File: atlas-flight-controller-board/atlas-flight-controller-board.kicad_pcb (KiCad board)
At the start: 4 copper layers, 55.6 x 67.6 mm, 36 parts, among them IC1 LSM6DSV80XTR, IC2 LPS22HHTR, J1 LED Indicator Header, J4 5V Input Power, U1 LIS2MDL, U2 DEV-16771, U3 746

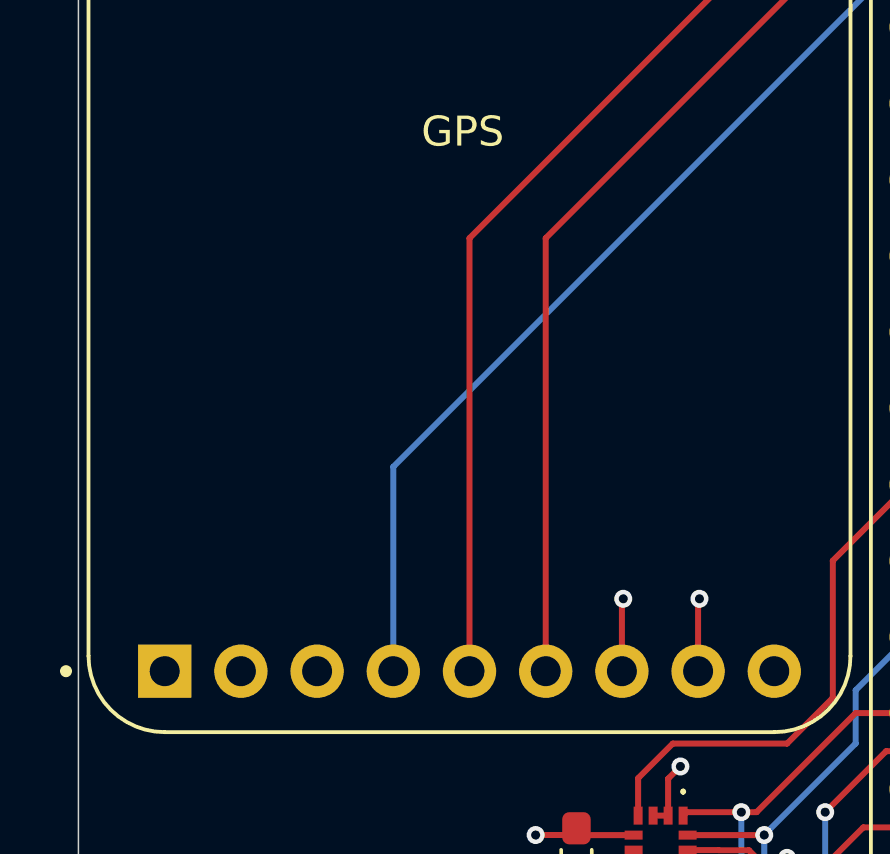
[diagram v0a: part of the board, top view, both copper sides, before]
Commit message: Test
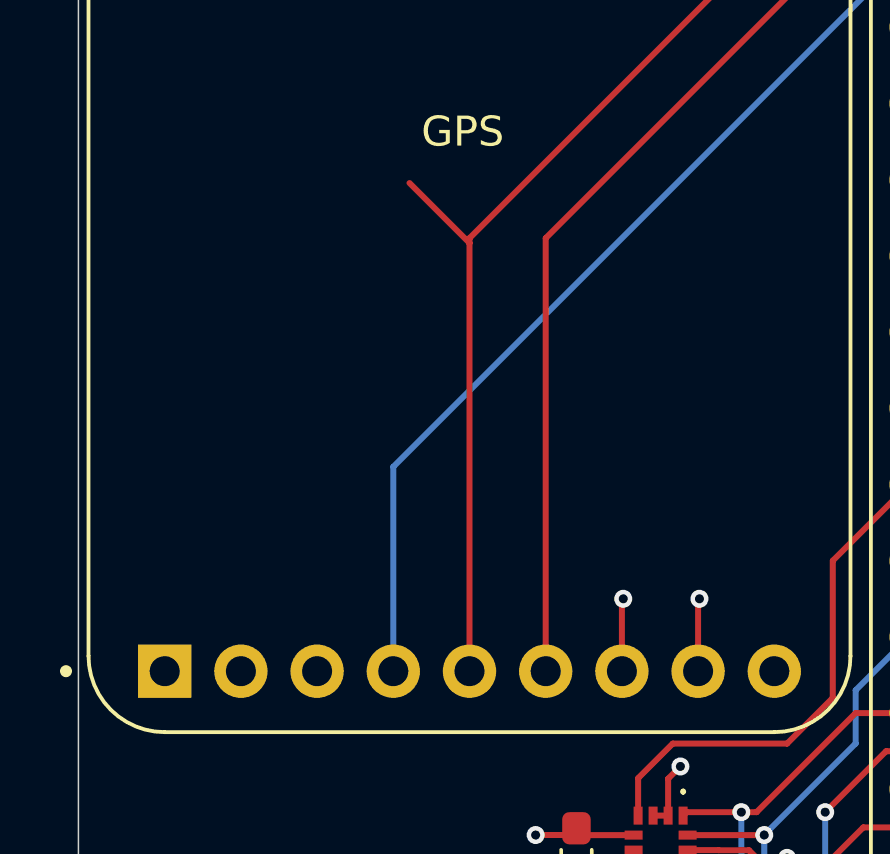
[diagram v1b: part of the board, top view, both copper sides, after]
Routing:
- net UART_GPS_TX_MCU_RX: track 35.2 -> 38.0 mm
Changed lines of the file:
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@@
 	)
 	(segment
-		(start 106 88.773)
+		(start 106 74.5)
 		(end 106 74.34)
+		(width 0.2)
+		(layer "F.Cu")
+		(net 9)
+	)
+	(segment
+		(start 106 74.5)
+		(end 104 72.5)
 		(width 0.2)
 		(layer "F.Cu")
@@
 		(width 0.2)
 		(layer "F.Cu")
+		(net 9)
+	)
+	(segment
+		(start 106 88.773)
+		(end 106 74.5)
+		(width 0.2)
+		(layer "F.Cu")

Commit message: testing commit on new branch made by kicad. branch name: version2
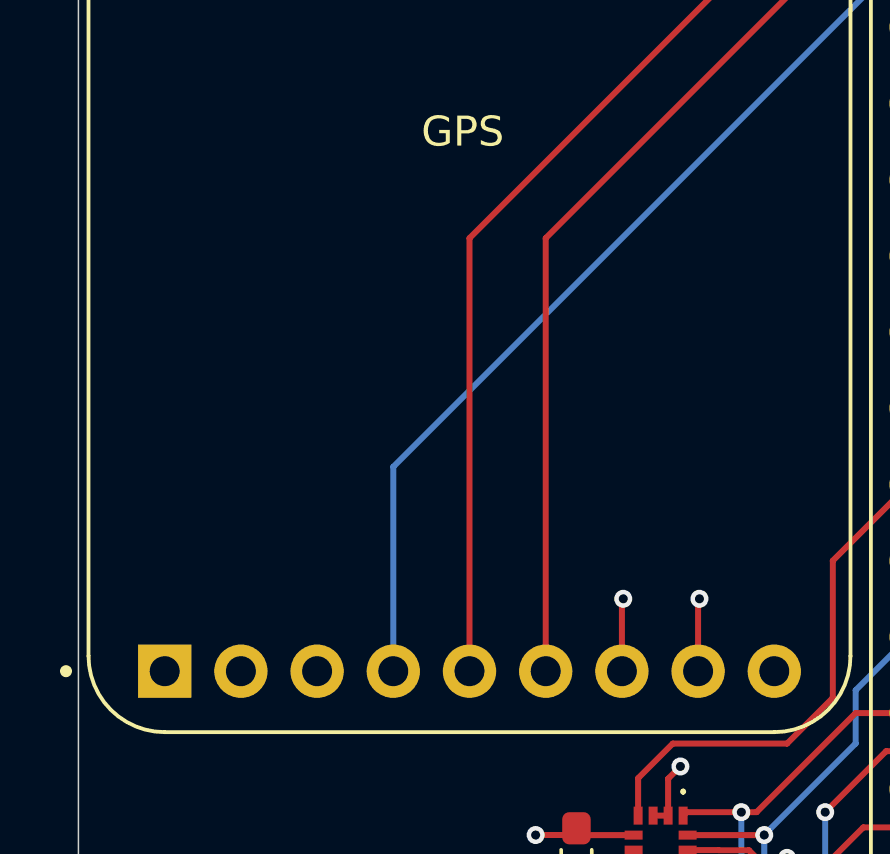
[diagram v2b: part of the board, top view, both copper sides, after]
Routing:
- net UART_GPS_TX_MCU_RX: track 38.0 -> 35.2 mm
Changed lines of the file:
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@@
 		(sheetname "/gps/")
 		(sheetfile "gps.kicad_sch")
-		(attr through_hole dnp)
+		(attr through_hole)
 		(fp_line
 			(start -12.7 14.605)
@@
 		(sheetname "/mcu-page/")
 		(sheetfile "mcu-page.kicad_sch")
-		(attr through_hole dnp)
+		(attr through_hole)
 		(fp_line
 			(start -30.48 8.89)
@@
 	)
 	(segment
-		(start 106 74.5)
+		(start 106 88.773)
 		(end 106 74.34)
 		(width 0.2)
@@
 	)
 	(segment
-		(start 106 74.5)
-		(end 104 72.5)
-		(width 0.2)
-		(layer "F.Cu")
-		(net 9)
-	)
-	(segment
 		(start 106 74.34)
 		(end 120.65 59.69)
 		(width 0.2)
 		(layer "F.Cu")
-		(net 9)
-	)
-	(segment
-		(start 106 88.773)
-		(end 106 74.5)
-		(width 0.2)
-		(layer "F.Cu")
